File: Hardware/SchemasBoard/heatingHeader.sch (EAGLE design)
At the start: 32 parts, among them IC1 DS1820, Q1 BSS84

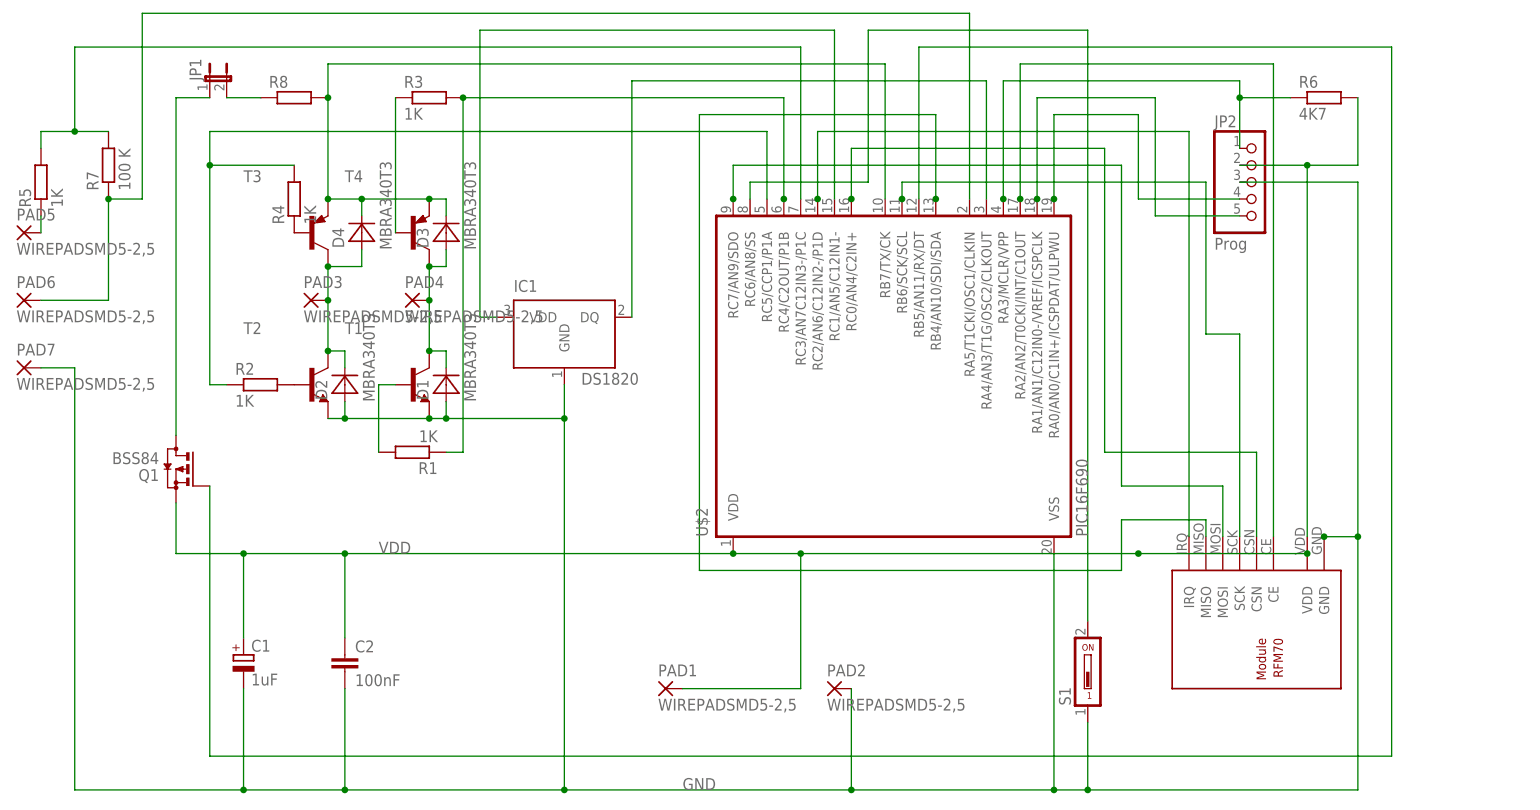
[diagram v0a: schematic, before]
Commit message: a
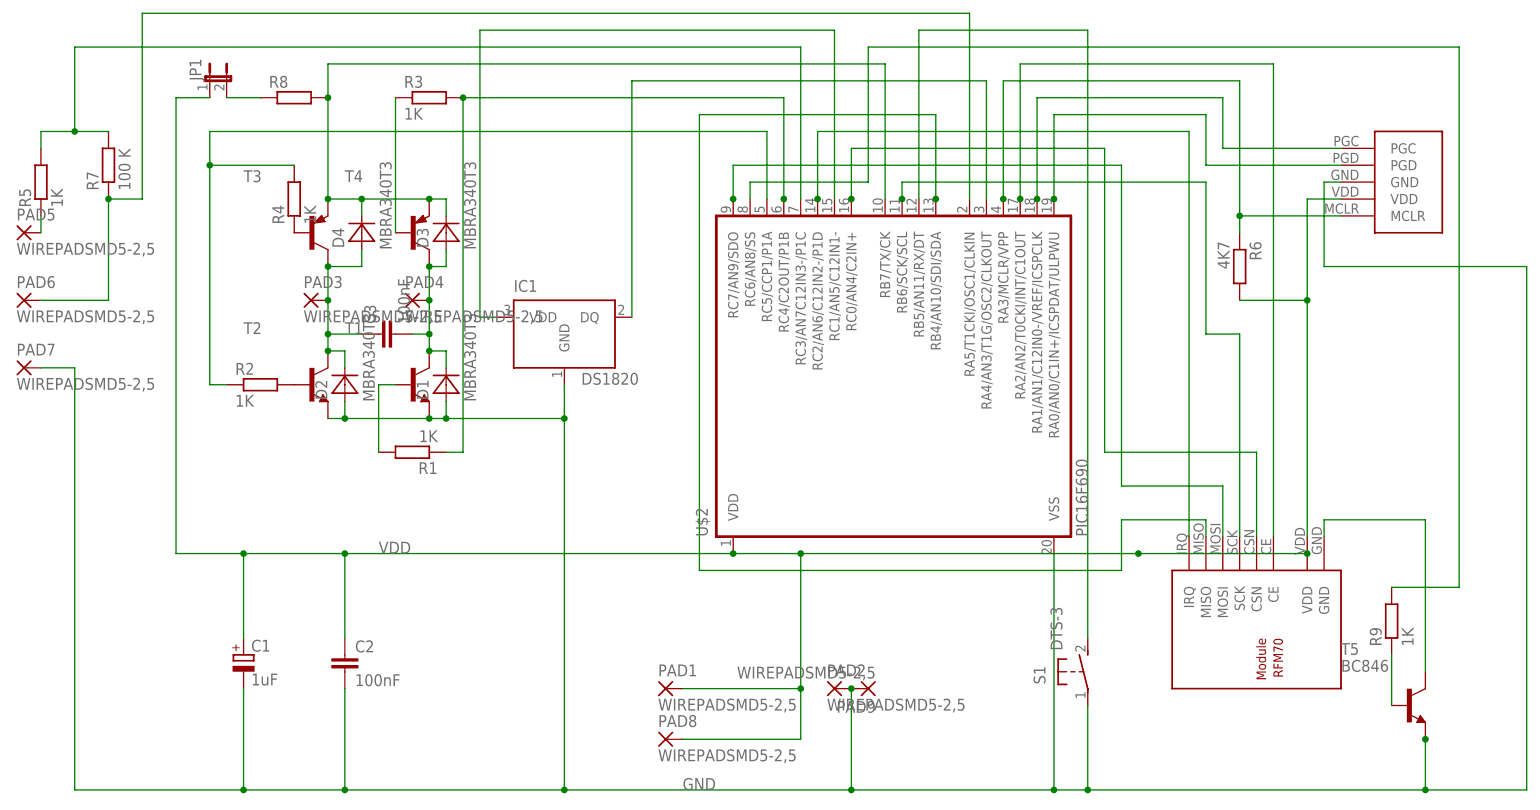
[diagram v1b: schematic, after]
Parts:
- removed JP2: Prog, pinhead:PINHD-1X5
- removed Q1: BSS84, transistor-small-signal:BSS84
- added C3: 100nF, resistor:C-EUC2012
- added PAD8, PAD9: WIREPADSMD5-2,5, wirepad:WIREPADSMD5-2,5
- added R9: 1K, resistor:R-EU_R1206
- added T5: BC846, transistor:BC846
- added U$3: PROGRAMMINGHEADERDIP, rfm70:PROGRAMMINGHEADERDIP
- S1: value (none) -> DTS-3; device switch-dil:SD4-01 -> switch-tact:DTS-3
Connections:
- new net N$5: R9.1, T5.B
- net GND: now also PAD9.P, T5.E, U$3.GND; no longer JP2.3, U$1.GND
- net N$10: now also U$2.RB5/AN11/RX/DT; no longer U$2.RC6/AN8/SS
- net N$11: now also R9.2, U$2.RC6/AN8/SS; no longer JP1.1, Q1.D
- net N$18: now also U$3.PGD; no longer JP2.4
- net N$19: now also U$3.PGC; no longer JP2.5
- net N$25: now also U$3.MCLR; no longer JP2.1
- net N$28: now also T5.C, U$1.GND; no longer Q1.G, U$2.RB5/AN11/RX/DT
- net N$7: now also C3.1
- net N$8: now also C3.2
- net VDD: now also JP1.1, PAD8.P, U$3.VDD; no longer JP2.2, Q1.S
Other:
- moved on the sheet: R6

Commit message: dfg
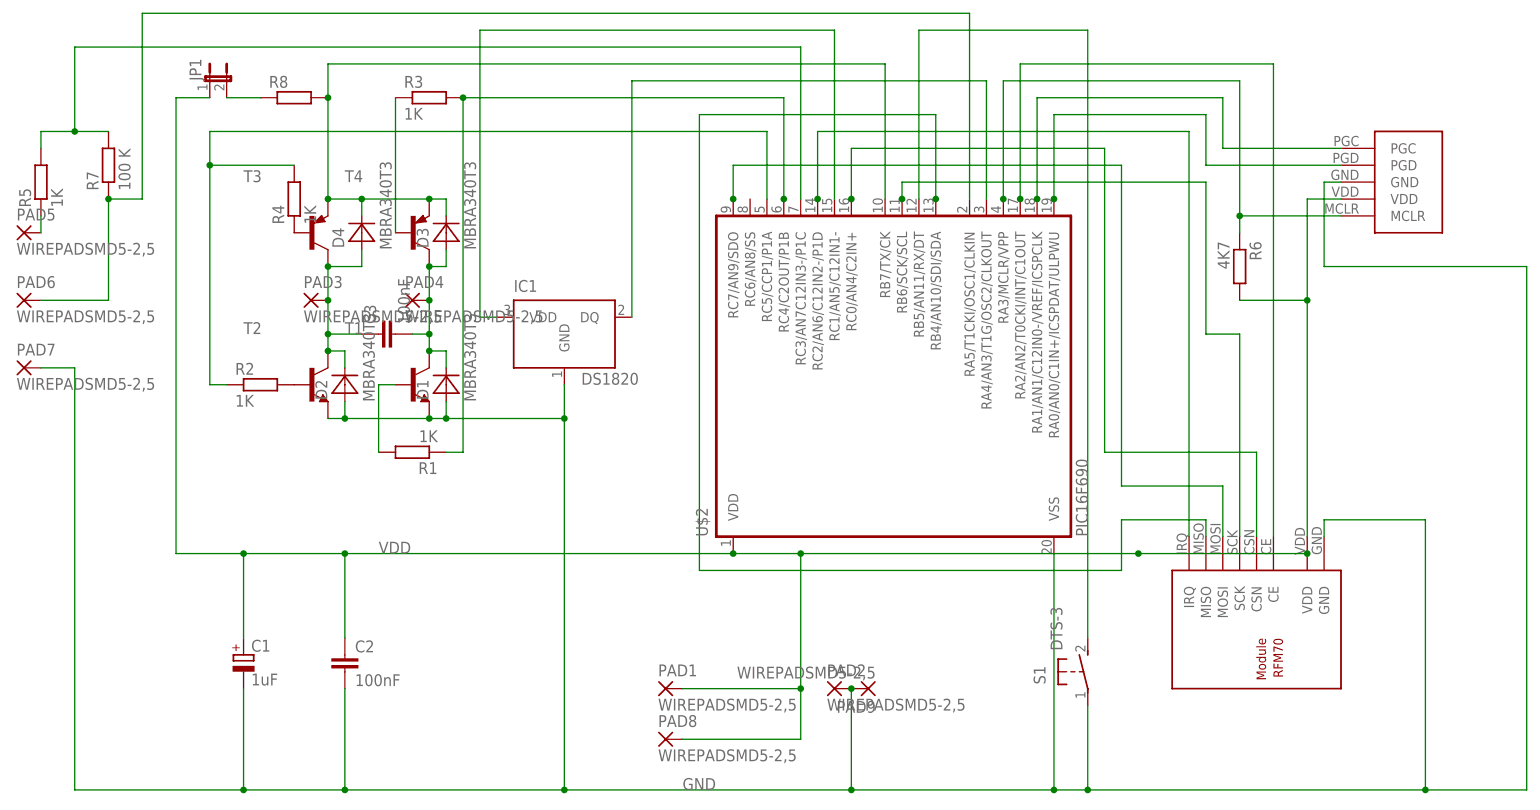
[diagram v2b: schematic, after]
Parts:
- removed R9: 1K, resistor:R-EU_R1206
- removed T5: BC846, transistor:BC846
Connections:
- removed net N$11: R9.2, U$2.RC6/AN8/SS
- removed net N$28: T5.C, U$1.GND
- removed net N$5: R9.1, T5.B
- net GND: now also U$1.GND; no longer T5.E
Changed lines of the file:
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@@
 <part name="R6" library="resistor" deviceset="R-EU_" device="R1206W" value="4K7"/>
 <part name="U$3" library="rfm70" deviceset="PROGRAMMINGHEADER" device="" technology="DIP"/>
-<part name="T5" library="transistor" deviceset="BC846" device=""/>
-<part name="R9" library="resistor" deviceset="R-EU_" device="R1206" value="1K"/>
 <part name="C3" library="resistor" deviceset="C-EU" device="C2012" value="100nF"/>
 <part name="PAD8" library="wirepad" deviceset="WIREPAD" device="SMD5-2,5"/>
@@
 <instance part="R6" gate="G$1" x="160.02" y="109.22" rot="R270"/>
 <instance part="U$3" gate="G$1" x="185.42" y="121.92"/>
-<instance part="T5" gate="G$1" x="185.42" y="43.18"/>
-<instance part="R9" gate="G$1" x="182.88" y="55.88" rot="R90"/>
 <instance part="C3" gate="G$1" x="30.48" y="99.06" rot="R90"/>
 <instance part="PAD8" gate="G$1" x="73.66" y="38.1"/>
@@
 <wire x1="132.08" y1="66.04" x2="132.08" y2="30.48" width="0.1524" layer="91"/>
 <pinref part="IC1" gate="G$1" pin="GND"/>
-<wire x1="187.96" y1="38.1" x2="187.96" y2="30.48" width="0.1524" layer="91"/>
 <wire x1="58.42" y1="91.44" x2="58.42" y2="86.36" width="0.1524" layer="91"/>
 <wire x1="58.42" y1="86.36" x2="58.42" y2="30.48" width="0.1524" layer="91"/>
@@
 <wire x1="203.2" y1="30.48" x2="187.96" y2="30.48" width="0.1524" layer="91"/>
 <junction x="187.96" y="30.48"/>
-<pinref part="T5" gate="G$1" pin="E"/>
-<junction x="187.96" y="38.1"/>
 <pinref part="PAD9" gate="G$1" pin="P"/>
 <junction x="101.6" y="45.72"/>
+<pinref part="U$1" gate="G$1" pin="GND"/>
+<wire x1="172.72" y1="71.12" x2="172.72" y2="68.58" width="0.1524" layer="91"/>
+<wire x1="187.96" y1="71.12" x2="172.72" y2="71.12" width="0.1524" layer="91"/>
+<wire x1="187.96" y1="71.12" x2="187.96" y2="30.48" width="0.1524" layer="91"/>
 </segment>
 </net>
@@
 </segment>
 </net>
-<net name="N$5" class="0">
-<segment>
-<pinref part="R9" gate="G$1" pin="1"/>
-<pinref part="T5" gate="G$1" pin="B"/>
-<wire x1="182.88" y1="50.8" x2="182.88" y2="43.18" width="0.1524" layer="91"/>
-</segment>
-</net>
-<net name="N$11" class="0">
-<segment>
-<pinref part="R9" gate="G$1" pin="2"/>
-<wire x1="182.88" y1="60.96" x2="193.04" y2="60.96" width="0.1524" layer="91"/>
-<wire x1="193.04" y1="60.96" x2="193.04" y2="142.24" width="0.1524" layer="91"/>
-<wire x1="193.04" y1="142.24" x2="104.14" y2="142.24" width="0.1524" layer="91"/>
-<wire x1="104.14" y1="142.24" x2="104.14" y2="121.92" width="0.1524" layer="91"/>
-<pinref part="U$2" gate="G$1" pin="RC6/AN8/SS"/>
-<wire x1="104.14" y1="121.92" x2="86.36" y2="121.92" width="0.1524" layer="91"/>
-<wire x1="86.36" y1="121.92" x2="86.36" y2="119.38" width="0.1524" layer="91"/>
-</segment>
-</net>
-<net name="N$28" class="0">
-<segment>
-<pinref part="U$1" gate="G$1" pin="GND"/>
-<wire x1="172.72" y1="71.12" x2="172.72" y2="68.58" width="0.1524" layer="91"/>
-<pinref part="T5" gate="G$1" pin="C"/>
-<wire x1="187.96" y1="48.26" x2="187.96" y2="71.12" width="0.1524" layer="91"/>
-<wire x1="187.96" y1="71.12" x2="172.72" y2="71.12" width="0.1524" layer="91"/>
-</segment>
-</net>
